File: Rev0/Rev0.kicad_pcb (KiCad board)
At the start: 2 copper layers, 71.7 x 72.8 mm, 142 parts, among them CON1 NA(NH1x20), J1 Conn_02x02_P4.20mm_Molex_Hori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, J2 Conn_01x04_P1.00mm_Stemma qt/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, J3 Conn_01x04_P1.00mm_Stemma qt/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, J4 Conn_01x04_P1.00mm_Stemma qt/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, J5 Conn_01x04_P1.00mm_Stemma qt/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, J6 Conn_01x04_P1.00mm_Stemma qt/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, J7 Conn_01x04_P1.00mm_Stemma qt/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, J8 Conn_01x04_P1.00mm_Stemma qt/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, J9 Conn_01x04_P1.00mm_Stemma qt/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, Q1 Q12MHz/20pF/30ppm/2P/HC-49SM(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, Q2 BC817-40(SOT23), Q3 BC817-40(SOT23), T1 DTC114YKA, U1 K7805-2000R3L, U2 CH340T(SSOP20W), U3 LAN8710A-EZC(QFN32), U4 K7803-2000R3L, U5 TCA9548APWR, U6 ESP32-WROOM-32D-4MB, U7 USB-C-16P-F(A40-00119-A52-12)

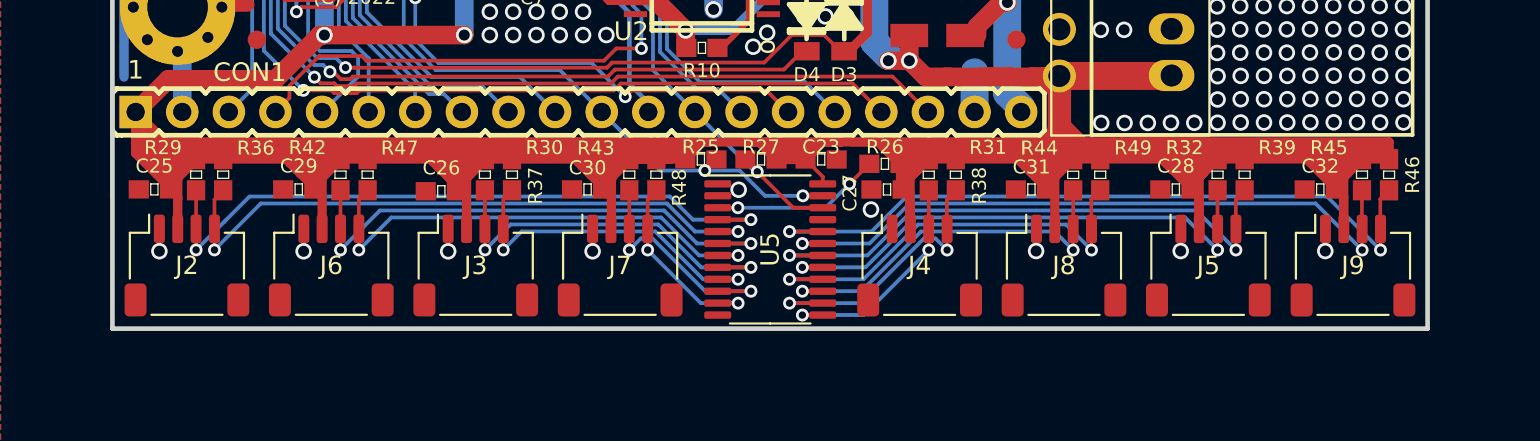
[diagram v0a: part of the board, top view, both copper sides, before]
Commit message: .
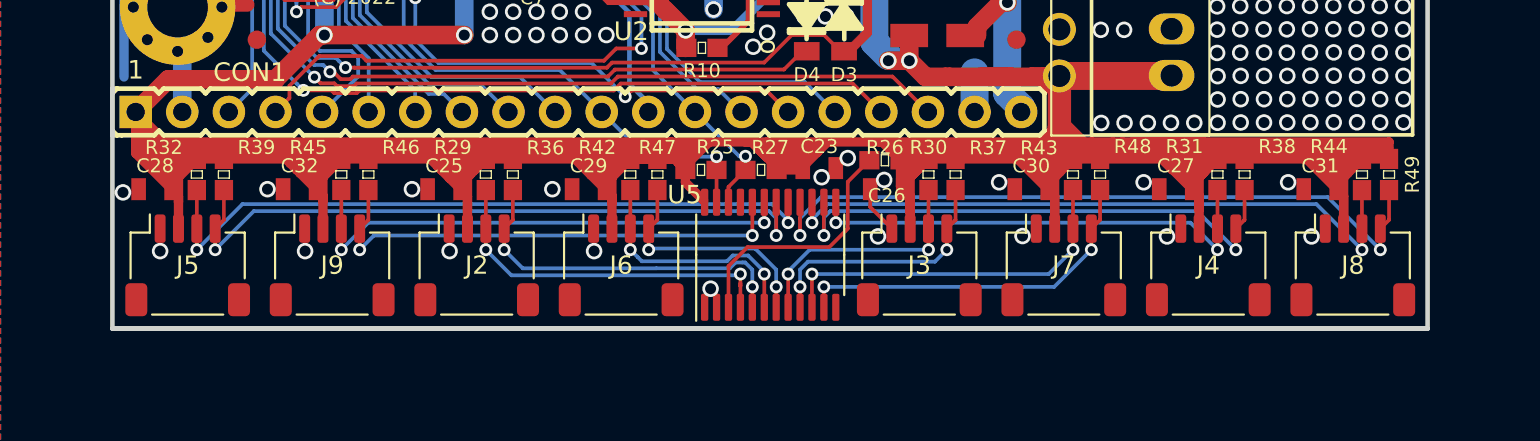
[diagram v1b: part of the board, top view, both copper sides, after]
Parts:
- C23: value 100nF/6.3V/20%/X5R/C0603 -> 100nF/6.3V/20%/X5R/C0805; footprint Capacitors:0603 -> Capacitors:0805
- C25, C26, C27, C28, C29, C30, C31, C32: value 1uF/6.3V/20%/X5R/C0603 -> 1uF/6.3V/20%/X5R/C0805; footprint Capacitors:0603 -> Capacitors:0805
- moved J9 55.6 mm to (81.6, 136.4)
- moved C28 55.6 mm to (71.9, 132.2)
- moved J5 55.6 mm to (73.7, 136.4)
- moved R32 55.6 mm to (74.2, 131.4)
- moved R39 55.6 mm to (75.7, 131.4)
- moved R46 55.6 mm to (83.5, 131.4)
- moved C32 55.6 mm to (79.8, 132.2)
- moved R45 55.6 mm to (82.1, 131.4)
- moved C26 24.3 mm to (111.8, 132.2)
- moved J7 24.2 mm to (121.5, 136.4)
- moved R43 24.2 mm to (122.0, 131.4)
- moved C30 24.2 mm to (119.7, 132.2)
- moved R48 24.2 mm to (123.4, 131.4)
- moved J3 24.2 mm to (113.6, 136.4)
- moved R30 24.2 mm to (114.1, 131.4)
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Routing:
- net Net-(J2-Pad3): track 37.2 -> 19.7 mm
- net Net-(J8-Pad4): track 23.9 -> 40.5 mm
- net Net-(J6-Pad3): track 29.1 -> 13.2 mm
- net Net-(J8-Pad3): track 21.3 -> 36.5 mm
- net Net-(J2-Pad4): track 34.8 -> 19.7 mm
- net Net-(J4-Pad4): track 16.0 -> 31.0 mm
- net Net-(J6-Pad4): track 26.8 -> 13.7 mm
- net Net-(J9-Pad4): track 39.9 -> 27.0 mm
- net Net-(J4-Pad3): track 13.1 -> 25.8 mm
- net +3V3: track 570.9 -> 582.5 mm
- net Net-(J5-Pad3): track 28.9 -> 38.1 mm
- net Net-(J7-Pad4): track 11.3 -> 20.5 mm
- net Net-(J9-Pad3): track 36.8 -> 28.0 mm
- net Net-(J3-Pad3): track 21.0 -> 13.7 mm
- net Net-(J7-Pad3): track 13.1 -> 20.2 mm
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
